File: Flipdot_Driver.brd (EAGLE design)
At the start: 160 x 100 mm, 28 parts

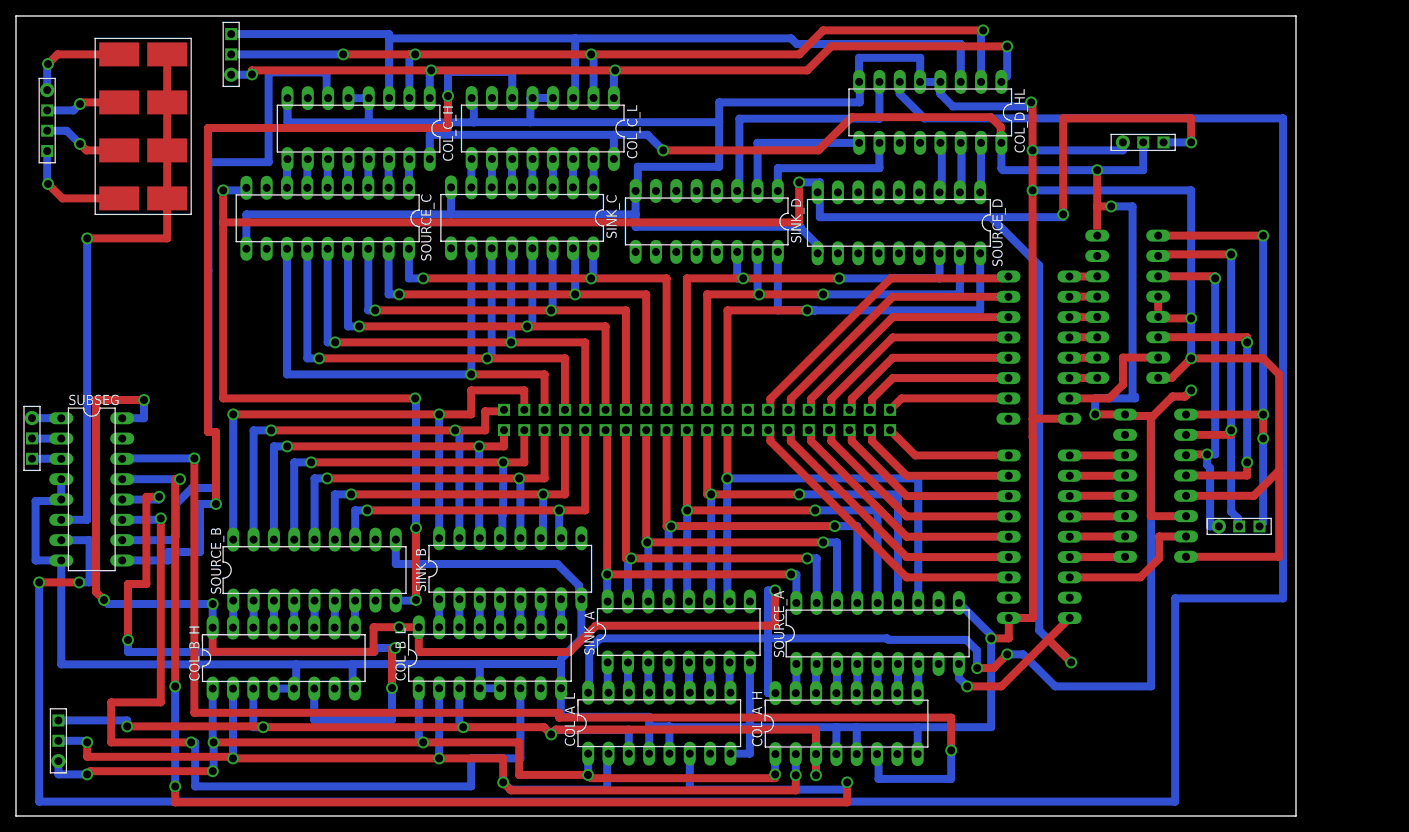
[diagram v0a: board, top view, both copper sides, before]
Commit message: Finished, sent for production review
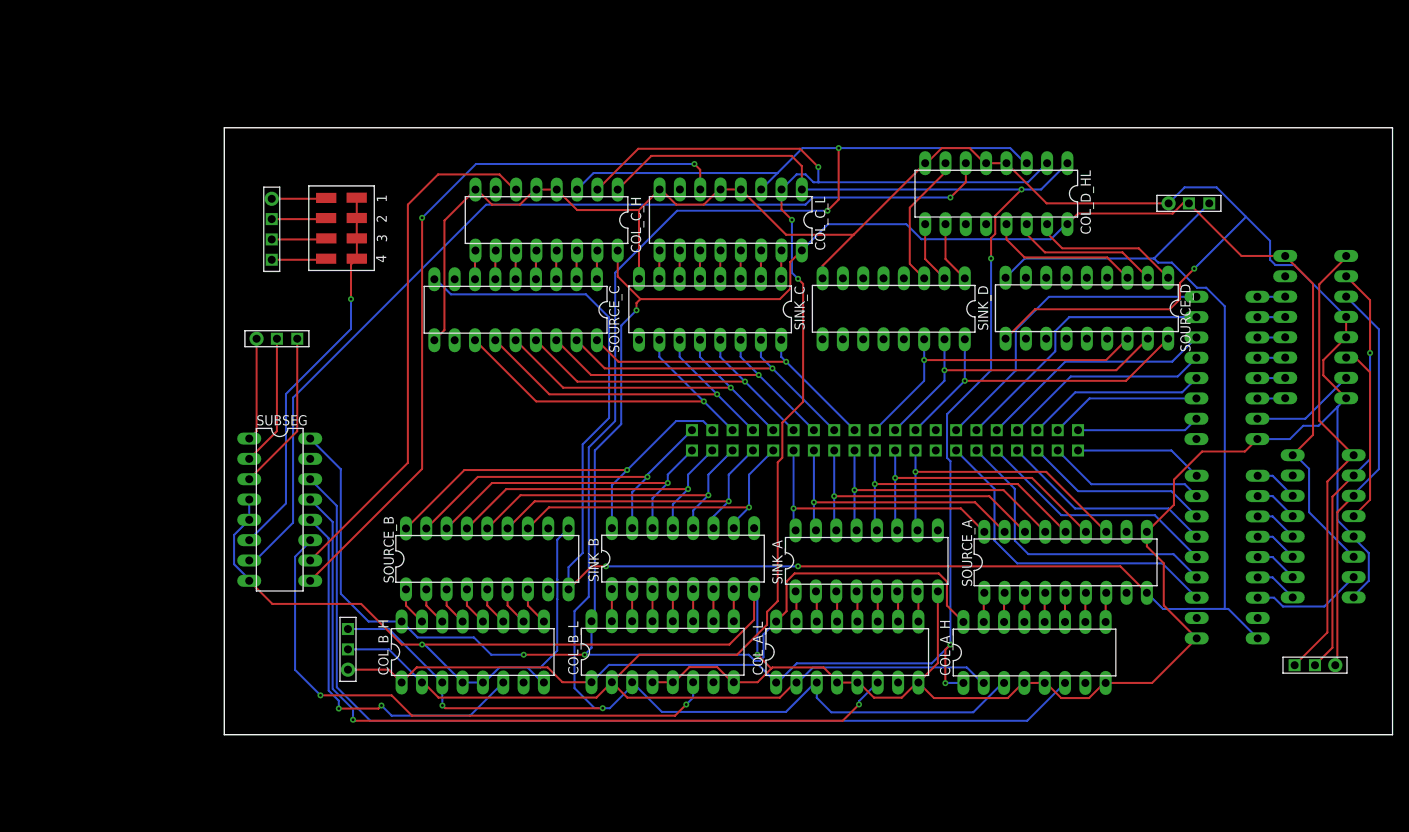
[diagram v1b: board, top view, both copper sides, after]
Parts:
- removed U$6: 3_PIN, Flipdot:3_PIN
- moved U$2 38.0 mm to (15.5, 10.8)
- moved U$3 33.1 mm to (6.62, 49.7), turned to 0 degrees
- moved U$11 31.2 mm to (5.97, 64.6)
- moved U$10 27.8 mm to (14.7, 63.5)
- moved COL_C_L 26.1 mm to (63.3, 64.5)
- moved SINK_C 26.1 mm to (60.8, 53.3)
- moved SOURCE_C 26.1 mm to (36.5, 53.3)
- moved COL_C_H 26.1 mm to (40.3, 64.5)
- moved SOURCE_D 25.8 mm to (107.9, 53.5)
- moved SINK_D 25.8 mm to (83.7, 53.4)
- moved COL_A_L 25.1 mm to (77.9, 10.5)
- moved SINK_A 25.1 mm to (80.3, 21.9)
- moved SOURCE_A 25.1 mm to (105.2, 21.7)
- moved COL_A_H 25.1 mm to (101.3, 10.4)
- moved COL_B_H 23.6 mm to (31.1, 10.5)
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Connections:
- net A: no longer U$6.P$1
- net B: no longer U$6.P$2
- net C: no longer U$6.P$3
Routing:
- net N$13: track 334.1 -> 120.7 mm, vias 2 -> 1
- net GND: track 685.9 -> 519.3 mm, vias 6 -> 3
- net 5V: track 456.0 -> 305.1 mm, vias 12 -> 3
- net 10V: track 313.9 -> 229.4 mm, vias 9 -> 2
- net N$7: track 159.8 -> 97.6 mm, vias 4 -> 2
- net N$8: track 85.2 -> 48.0 mm, vias 4 -> 2
- net N$10: track 108.1 -> 72.0 mm
- net N$9: track 156.1 -> 122.1 mm, vias 2 -> 0
- net C1: track 61.2 -> 37.0 mm
- net N$12: track 115.1 -> 91.5 mm
- net SEG_1: track 71.4 -> 48.4 mm
- net N$11: track 87.8 -> 65.4 mm
- net C3: track 59.1 -> 36.7 mm, vias 2 -> 1
- net C2: track 63.1 -> 41.5 mm
- net C20: track 68.1 -> 46.9 mm
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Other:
- board size 160 x 100 mm -> 146 x 75.9 mm
- board text added: "GND 5V 10V"
- board text added: "MCU 2 3 4"
- board text added: "MCU 5 6 7"
- board text added: "MCU 8 9 10"
- board text added: "Seg. Sel."
- board text added: "The cake is a lie."
